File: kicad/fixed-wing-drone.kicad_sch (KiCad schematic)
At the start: 25 parts, among them J1 1, J10 ACC POWER, J11 RC POWER, J12 Airspeed I2C, J13 EXTRA STEMMA QT, J14 QT I2C, J15 QT I2C, J17 FC UBEC Input, J18 ESC UBEC Input, J19 Secondary ESC, J2 2, J20 LIDAR BKUP, J21 AUX, J3 3, J4 4, J5 5, J6 6, J7 RC SIGNAL IN, J8 LIDAR, J9 GPS, Q1 FC REV POLARITY PROT, Q2 ESC REV POLARITY PROT, U1 ESP32-S3-DevKitC

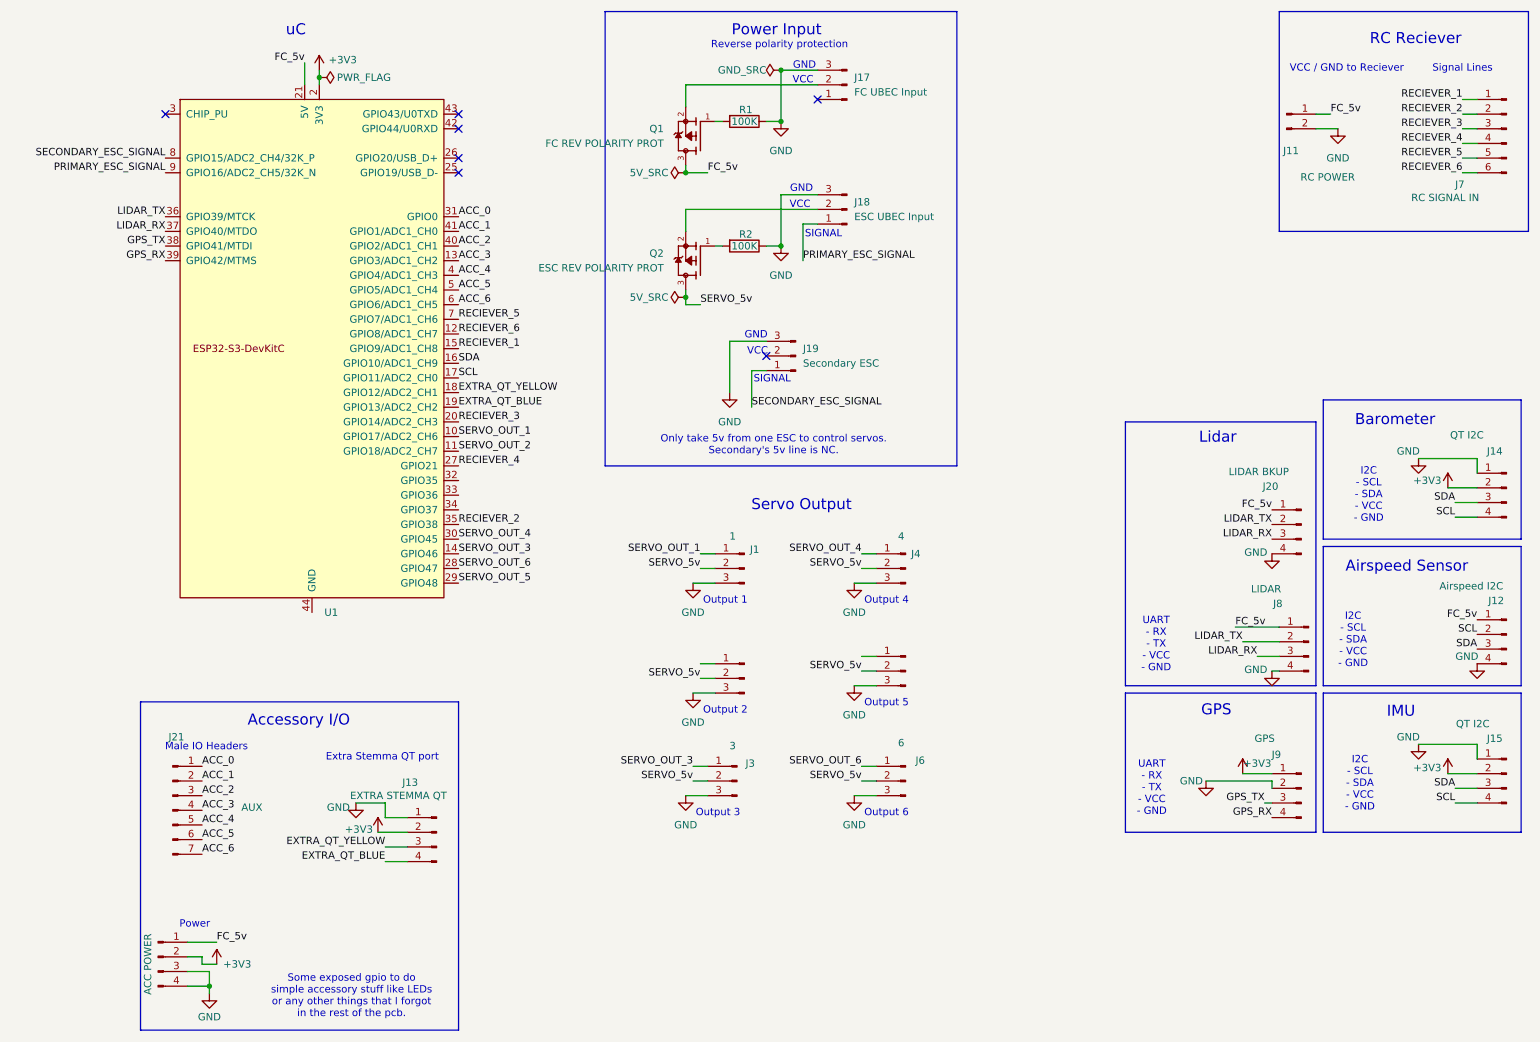
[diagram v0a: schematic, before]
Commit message: PCB v3.0
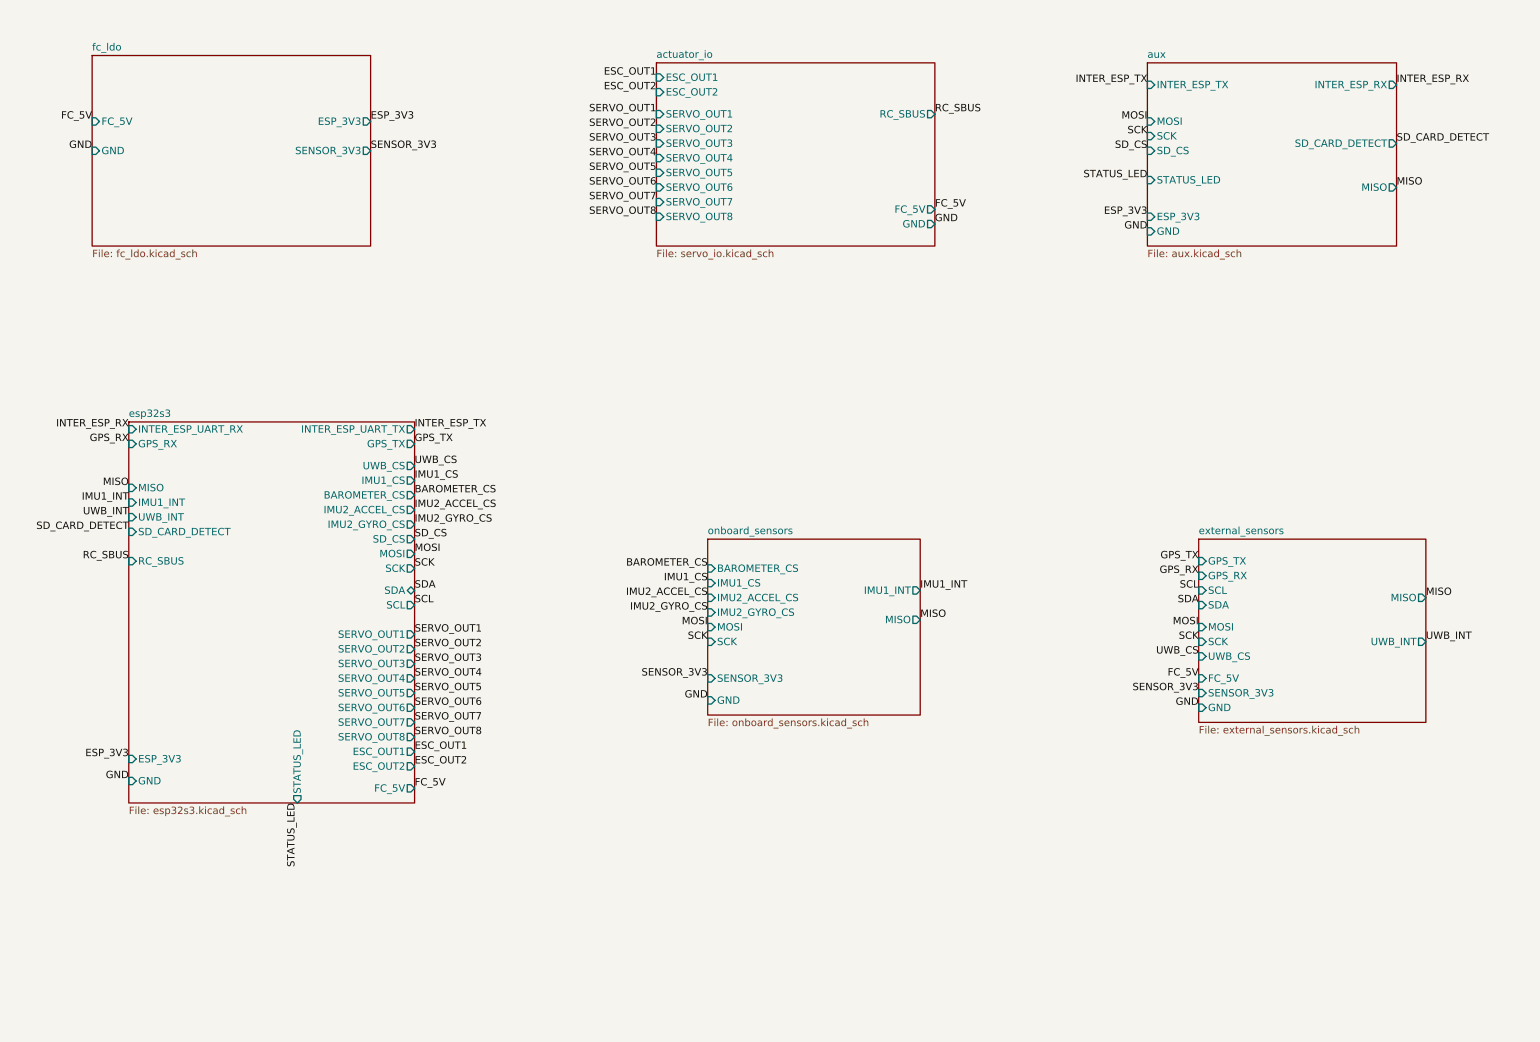
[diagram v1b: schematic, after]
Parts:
- removed J1: 1, Connector_PinHeader_2.54mm:PinHeader_1x03_P2.54mm_Vertical, symbol Connector:Conn_01x03_Pin
- removed J10: ACC POWER, Connector_PinHeader_2.54mm:PinHeader_1x04_P2.54mm_Vertical, symbol Connector:Conn_01x04_Pin
- removed J11: RC POWER, Connector_PinHeader_2.54mm:PinHeader_1x02_P2.54mm_Vertical, symbol Connector:Conn_01x02_Pin
- removed J12: Airspeed I2C, Connector_JST:JST_GH_BM04B-GHS-TBT_1x04-1MP_P1.25mm_Vertical, symbol Connector:Conn_01x04_Pin
- removed J13: EXTRA STEMMA QT, Connector_JST:JST_SH_BM04B-SRSS-TB_1x04-1MP_P1.00mm_Vertical, symbol Connector:Conn_01x04_Pin
- removed J14, J15: QT I2C, Connector_JST:JST_SH_BM04B-SRSS-TB_1x04-1MP_P1.00mm_Vertical, symbol Connector:Conn_01x04_Pin
- removed J17: FC UBEC Input, Connector_PinHeader_2.54mm:PinHeader_1x03_P2.54mm_Vertical, symbol Connector:Conn_01x03_Pin
- removed J18: ESC UBEC Input, Connector_PinHeader_2.54mm:PinHeader_1x03_P2.54mm_Vertical, symbol Connector:Conn_01x03_Pin
- removed J19: Secondary ESC, Connector_PinHeader_2.54mm:PinHeader_1x03_P2.54mm_Vertical, symbol Connector:Conn_01x03_Pin
- removed J2: 2, Connector_PinHeader_2.54mm:PinHeader_1x03_P2.54mm_Vertical, symbol Connector:Conn_01x03_Pin
- removed J20: LIDAR BKUP, Connector_PinHeader_2.54mm:PinHeader_1x04_P2.54mm_Vertical, symbol Connector:Conn_01x04_Pin
- removed J21: AUX, Connector_PinHeader_2.54mm:PinHeader_1x07_P2.54mm_Vertical, symbol Connector:Conn_01x07_Pin
- removed J3: 3, Connector_PinHeader_2.54mm:PinHeader_1x03_P2.54mm_Vertical, symbol Connector:Conn_01x03_Pin
- removed J4: 4, Connector_PinHeader_2.54mm:PinHeader_1x03_P2.54mm_Vertical, symbol Connector:Conn_01x03_Pin
- removed J5: 5, Connector_PinHeader_2.54mm:PinHeader_1x03_P2.54mm_Vertical, symbol Connector:Conn_01x03_Pin
- removed J6: 6, Connector_PinHeader_2.54mm:PinHeader_1x03_P2.54mm_Vertical, symbol Connector:Conn_01x03_Pin
- removed J7: RC SIGNAL IN, Connector_PinHeader_2.54mm:PinHeader_1x06_P2.54mm_Vertical, symbol Connector:Conn_01x06_Pin
- removed J8: LIDAR, Connector_Molex:Molex_PicoBlade_53398-0471_1x04-1MP_P1.25mm_Vertical, symbol Connector:Conn_01x04_Pin
- removed J9: GPS, Connector_PinHeader_2.54mm:PinHeader_1x04_P2.54mm_Vertical, symbol Connector:Conn_01x04_Pin
- removed Q1: FC REV POLARITY PROT, AO3407A:SOT95P280X125-3N, symbol AO3407A:AO3407A
- removed Q2: ESC REV POLARITY PROT, AO3407A:SOT95P280X125-3N, symbol AO3407A:AO3407A
- removed R1, R2: 100K, Resistor_SMD:R_0402_1005Metric, symbol Device:R
- removed U1: ESP32-S3-DevKitC, PCM_Espressif:ESP32-S3-DevKitC-trav-snf2, symbol PCM_Espressif:ESP32-S3-DevKitC
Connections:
- no-connect marks 7 -> 0
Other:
- added sheet actuator_io (servo_io.kicad_sch)
- added sheet aux (aux.kicad_sch)
- added sheet esp32s3 (esp32s3.kicad_sch)
- added sheet external_sensors (external_sensors.kicad_sch)
- added sheet fc_ldo (fc_ldo.kicad_sch)
- added sheet onboard_sensors (onboard_sensors.kicad_sch)
- note removed: "Accessory I/O"
- note removed: "Airspeed Sensor"
- note removed: "Barometer"
- note removed: "Extra Stemma QT port"
- note removed: "GND"
- note removed: "GPS"
- note removed: "I2C - SCL - SDA - VCC - GND"
- note removed: "IMU"
- note removed: "Lidar"
- note removed: "Male IO Headers"
- note removed: "Only take 5v from one ESC to control servos. Secondary's 5v line is NC."
- note removed: "Output 1"
- note removed: "Output 2"
- note removed: "Output 3"
- note removed: "Output 4"
- note removed: "Output 5"
- note removed: "Output 6"
- note removed: "Power"
- note removed: "Power Input"
- note removed: "RC Reciever"
- note removed: "Reverse polarity protection"
- note removed: "SIGNAL"
- note removed: "Servo Output"
- note removed: "Signal Lines"
- note removed: "Some exposed gpio to do simple accessory stuff like LEDs or any other things that I forgot in the rest of the pcb."
- note removed: "UART - RX - TX - VCC - GND"
- note removed: "VCC"
- note removed: "VCC / GND to Reciever"
- note removed: "uC"
